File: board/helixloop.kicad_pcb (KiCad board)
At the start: 2 copper layers, 136.7 x 136.7 mm, 374 parts, among them J1 Conn_01x04, J2 Conn_01x02

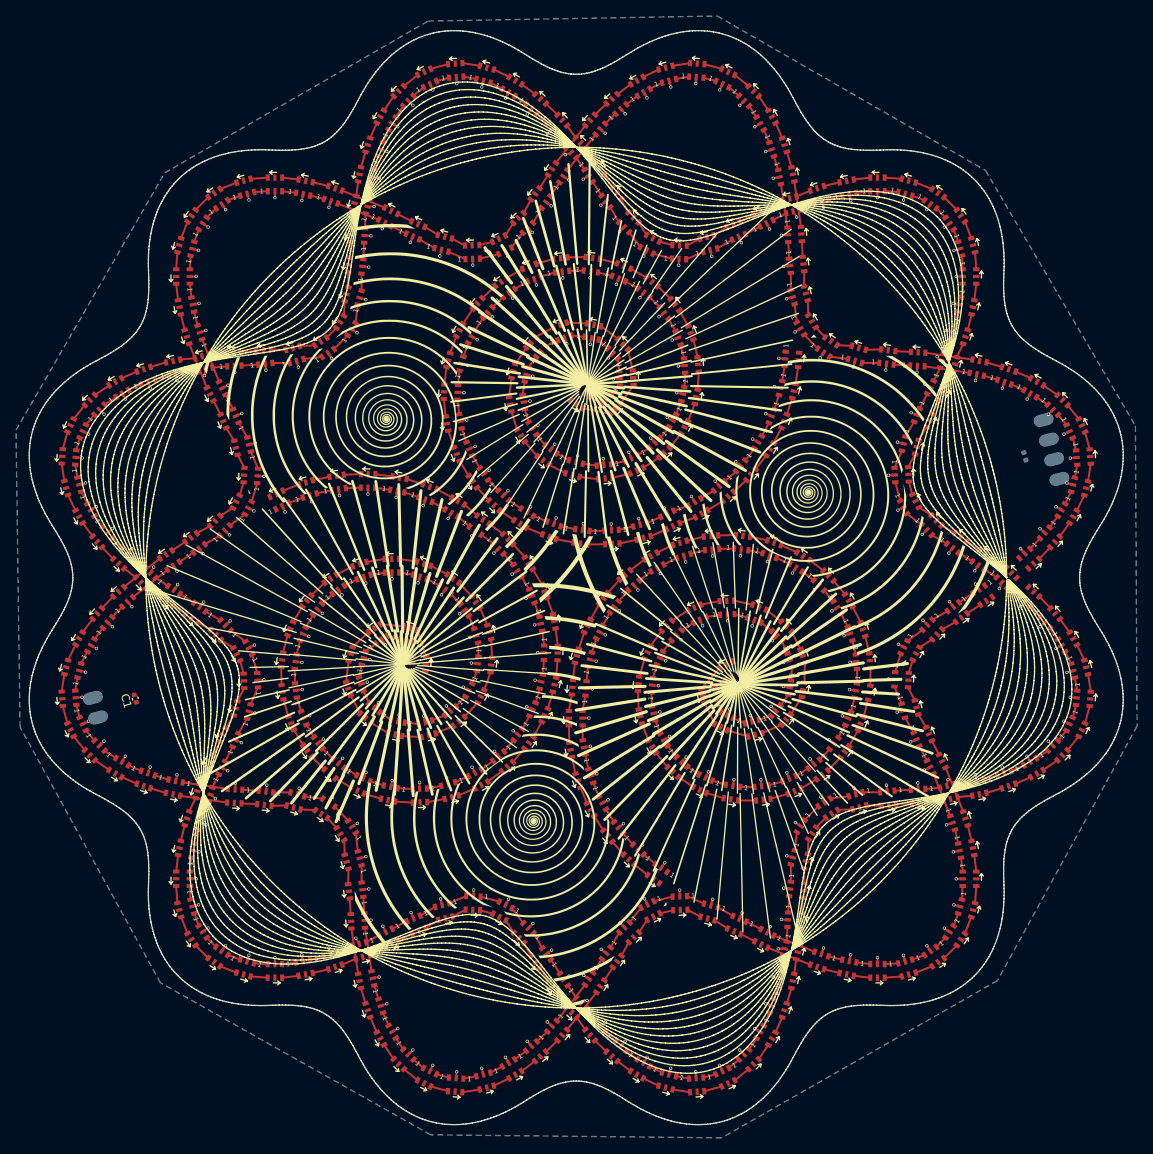
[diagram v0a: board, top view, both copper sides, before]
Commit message: draft routing
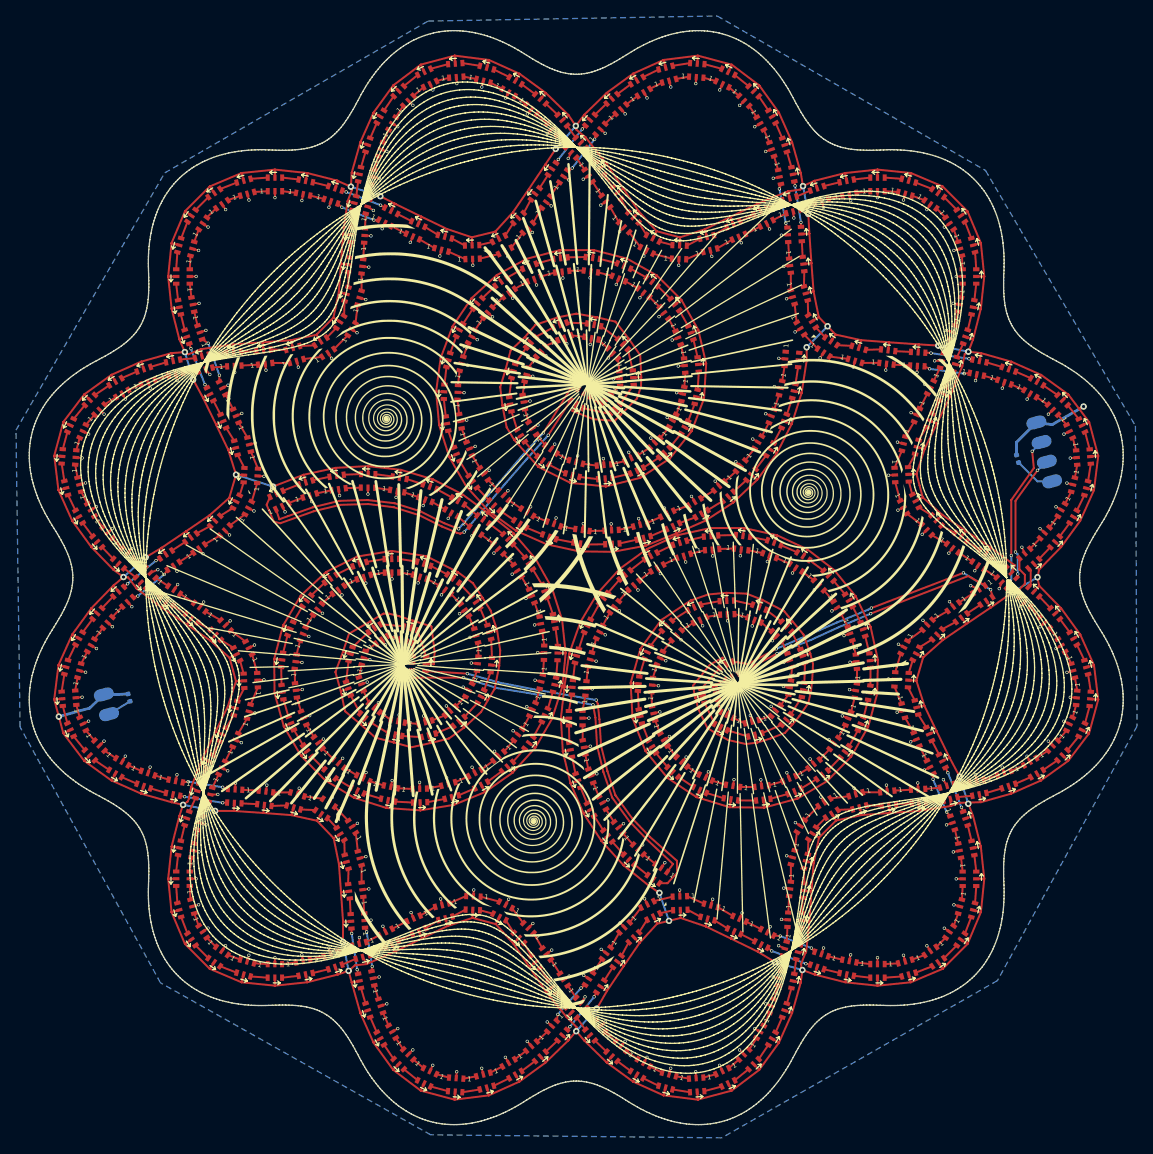
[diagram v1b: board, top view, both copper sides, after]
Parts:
- C1: moved to B.Cu
- D1, D10, D100, D101, D102, D103, D104, D105, D106, D107, D108, D109, D11, D110, D111, D112, D113, D114, D115, D116, D117, D118, D119, D12, D120, D121, D122, D123, D124, D125, D126, D127, D128, D129, D13, D130, D131, D132, D133, D134, D135, D136, D137, D138, D139, D14, D140, D141, D142, D143, D144, D145, D146, D147, D148, D149, D15, D150, D151, D152, D153, D154, D155, D156, D157, D158, D159, D16, D160, D161, D162, D163, D164, D165, D166, D167, D168, D169, D17, D170, D171, D172, D173, D174, D175, D176, D177, D178, D179, D18, D180, D181, D182, D183, D184, D185, D186, D187, D188, D189, D19, D190, D191, D192, D193, D194, D195, D196, D197, D198, D199, D2, D20, D200, D201, D202, D203, D204, D205, D206, D207, D208, D209, D21, D210, D211, D212, D213, D214, D215, D216, D217, D218, D219, D22, D220, D221, D222, D223, D224, D225, D226, D227, D228, D229, D23, D230, D231, D232, D233, D234, D235, D236, D237, D238, D239, D24, D240, D241, D242, D243, D244, D245, D246, D247, D248, D249, D25, D250, D251, D252, D253, D254, D255, D256, D257, D258, D259, D26, D260, D261, D262, D263, D264, D265, D266, D267, D268, D269, D27, D270, D271, D272, D273, D274, D275, D276, D277, D278, D279, D28, D280, D281, D282, D283, D284, D285, D286, D287, D288, D289, D29, D290, D291, D292, D293, D294, D295, D296, D297, D298, D299, D3, D30, D300, D301, D302, D303, D304, D305, D306, D307, D308, D309, D31, D310, D311, D312, D313, D314, D315, D316, D317, D318, D319, D32, D320, D321, D322, D323, D324, D325, D326, D327, D328, D329, D33, D330, D331, D332, D333, D334, D335, D336, D337, D338, D339, D34, D340, D341, D342, D343, D344, D345, D346, D347, D348, D349, D35, D350, D351, D352, D353, D354, D355, D356, D357, D358, D359, D36, D360, D361, D362, D363, D364, D365, D366, D367, D368, D369, D37, D38, D39, D4, D40, D41, D42, D43, D44, D45, D46, D47, D48, D49, D5, D50, D51, D52, D53, D54, D55, D56, D57, D58, D59, D6, D60, D61, D62, D63, D64, D65, D66, D67, D68, D69, D7, D70, D71, D72, D73, D74, D75, D76, D77, D78, D79, D8, D80, D81, D82, D83, D84, D85, D86, D87, D88, D89, D9, D90, D91, D92, D93, D94, D95, D96, D97, D98, D99: value LED-SK9822-EC20 -> SK9822-EC20
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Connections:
- D1 pad 1: (no net) -> Net-(D1-Pad1)
- D1 pad 2: (no net) -> GND
- D1 pad 3: (no net) -> /LED_SDI1
- D1 pad 4: (no net) -> /LED_CKI1
- D1 pad 5: (no net) -> +5V
- D1 pad 6: (no net) -> Net-(D1-Pad6)
- D10 pad 1: (no net) -> Net-(D10-Pad1)
- D10 pad 2: (no net) -> GND
- D10 pad 3: (no net) -> Net-(D10-Pad3)
- D10 pad 4: (no net) -> Net-(D10-Pad4)
- D10 pad 5: (no net) -> +5V
- D10 pad 6: (no net) -> Net-(D10-Pad6)
- D100 pad 1: (no net) -> Net-(D100-Pad1)
- D100 pad 2: (no net) -> GND
- D100 pad 3: (no net) -> Net-(D100-Pad3)
- D100 pad 4: (no net) -> Net-(D100-Pad4)
- D100 pad 5: (no net) -> +5V
- D100 pad 6: (no net) -> Net-(D100-Pad6)
- D101 pad 1: (no net) -> Net-(D101-Pad1)
- D101 pad 2: (no net) -> GND
- D101 pad 3: (no net) -> Net-(D100-Pad1)
- D101 pad 4: (no net) -> Net-(D100-Pad6)
- D101 pad 5: (no net) -> +5V
- D101 pad 6: (no net) -> Net-(D101-Pad6)
- D102 pad 1: (no net) -> Net-(D102-Pad1)
- D102 pad 2: (no net) -> GND
- D102 pad 3: (no net) -> Net-(D101-Pad1)
- D102 pad 4: (no net) -> Net-(D101-Pad6)
- D102 pad 5: (no net) -> +5V
- D102 pad 6: (no net) -> Net-(D102-Pad6)
- D103 pad 1: (no net) -> Net-(D103-Pad1)
- D103 pad 2: (no net) -> GND
- D103 pad 3: (no net) -> Net-(D102-Pad1)
- D103 pad 4: (no net) -> Net-(D102-Pad6)
- D103 pad 5: (no net) -> +5V
- D103 pad 6: (no net) -> Net-(D103-Pad6)
- D104 pad 1: (no net) -> Net-(D104-Pad1)
- D104 pad 2: (no net) -> GND
- D104 pad 3: (no net) -> Net-(D103-Pad1)
- D104 pad 4: (no net) -> Net-(D103-Pad6)
- D104 pad 5: (no net) -> +5V
- D104 pad 6: (no net) -> Net-(D104-Pad6)
- D105 pad 1: (no net) -> Net-(D105-Pad1)
- D105 pad 2: (no net) -> GND
- D105 pad 3: (no net) -> Net-(D104-Pad1)
- D105 pad 4: (no net) -> Net-(D104-Pad6)
- D105 pad 5: (no net) -> +5V
- D105 pad 6: (no net) -> Net-(D105-Pad6)
- D106 pad 1: (no net) -> Net-(D106-Pad1)
- D106 pad 2: (no net) -> GND
- D106 pad 3: (no net) -> Net-(D105-Pad1)
- D106 pad 4: (no net) -> Net-(D105-Pad6)
- D106 pad 5: (no net) -> +5V
- D106 pad 6: (no net) -> Net-(D106-Pad6)
- D107 pad 1: (no net) -> Net-(D107-Pad1)
- D107 pad 2: (no net) -> GND
- D107 pad 3: (no net) -> Net-(D106-Pad1)
- D107 pad 4: (no net) -> Net-(D106-Pad6)
- D107 pad 5: (no net) -> +5V
- D107 pad 6: (no net) -> Net-(D107-Pad6)
- D108 pad 1: (no net) -> Net-(D108-Pad1)
- D108 pad 2: (no net) -> GND
- D108 pad 3: (no net) -> Net-(D107-Pad1)
- D108 pad 4: (no net) -> Net-(D107-Pad6)
- D108 pad 5: (no net) -> +5V
- D108 pad 6: (no net) -> Net-(D108-Pad6)
- D109 pad 1: (no net) -> Net-(D109-Pad1)
- D109 pad 2: (no net) -> GND
- D109 pad 3: (no net) -> Net-(D108-Pad1)
- D109 pad 4: (no net) -> Net-(D108-Pad6)
- D109 pad 5: (no net) -> +5V
- D109 pad 6: (no net) -> Net-(D109-Pad6)
- D11 pad 1: (no net) -> Net-(D11-Pad1)
- D11 pad 2: (no net) -> GND
- D11 pad 3: (no net) -> Net-(D10-Pad1)
- D11 pad 4: (no net) -> Net-(D10-Pad6)
- D11 pad 5: (no net) -> +5V
- D11 pad 6: (no net) -> Net-(D11-Pad6)
- D110 pad 1: (no net) -> Net-(D110-Pad1)
- D110 pad 2: (no net) -> GND
- D110 pad 3: (no net) -> Net-(D109-Pad1)
- D110 pad 4: (no net) -> Net-(D109-Pad6)
- D110 pad 5: (no net) -> +5V
- D110 pad 6: (no net) -> Net-(D110-Pad6)
- D111 pad 1: (no net) -> Net-(D111-Pad1)
- D111 pad 2: (no net) -> GND
- D111 pad 3: (no net) -> Net-(D110-Pad1)
- D111 pad 4: (no net) -> Net-(D110-Pad6)
- D111 pad 5: (no net) -> +5V
- D111 pad 6: (no net) -> Net-(D111-Pad6)
- D112 pad 1: (no net) -> Net-(D112-Pad1)
- D112 pad 2: (no net) -> GND
- D112 pad 3: (no net) -> Net-(D111-Pad1)
- D112 pad 4: (no net) -> Net-(D111-Pad6)
- D112 pad 5: (no net) -> +5V
- D112 pad 6: (no net) -> Net-(D112-Pad6)
- D113 pad 1: (no net) -> Net-(D113-Pad1)
- D113 pad 2: (no net) -> GND
- D113 pad 3: (no net) -> Net-(D112-Pad1)
- D113 pad 4: (no net) -> Net-(D112-Pad6)
- D113 pad 5: (no net) -> +5V
- D113 pad 6: (no net) -> Net-(D113-Pad6)
- D114 pad 1: (no net) -> Net-(D114-Pad1)
- D114 pad 2: (no net) -> GND
- D114 pad 3: (no net) -> Net-(D113-Pad1)
- D114 pad 4: (no net) -> Net-(D113-Pad6)
- D114 pad 5: (no net) -> +5V
- D114 pad 6: (no net) -> Net-(D114-Pad6)
- D115 pad 1: (no net) -> Net-(D115-Pad1)
- D115 pad 2: (no net) -> GND
- D115 pad 3: (no net) -> Net-(D114-Pad1)
- D115 pad 4: (no net) -> Net-(D114-Pad6)
- D115 pad 5: (no net) -> +5V
- D115 pad 6: (no net) -> Net-(D115-Pad6)
- D116 pad 1: (no net) -> Net-(D116-Pad1)
- D116 pad 2: (no net) -> GND
- D116 pad 3: (no net) -> Net-(D115-Pad1)
- D116 pad 4: (no net) -> Net-(D115-Pad6)
- D116 pad 5: (no net) -> +5V
- D116 pad 6: (no net) -> Net-(D116-Pad6)
- D117 pad 1: (no net) -> Net-(D117-Pad1)
- D117 pad 2: (no net) -> GND
- D117 pad 3: (no net) -> Net-(D116-Pad1)
- D117 pad 4: (no net) -> Net-(D116-Pad6)
- D117 pad 5: (no net) -> +5V
- D117 pad 6: (no net) -> Net-(D117-Pad6)
- D118 pad 1: (no net) -> Net-(D118-Pad1)
- D118 pad 2: (no net) -> GND
- D118 pad 3: (no net) -> Net-(D117-Pad1)
- D118 pad 4: (no net) -> Net-(D117-Pad6)
- D118 pad 5: (no net) -> +5V
- D118 pad 6: (no net) -> Net-(D118-Pad6)
- D119 pad 1: (no net) -> Net-(D119-Pad1)
- D119 pad 2: (no net) -> GND
- D119 pad 3: (no net) -> Net-(D118-Pad1)
- D119 pad 4: (no net) -> Net-(D118-Pad6)
- D119 pad 5: (no net) -> +5V
- D119 pad 6: (no net) -> Net-(D119-Pad6)
- D12 pad 1: (no net) -> Net-(D12-Pad1)
- D12 pad 2: (no net) -> GND
- D12 pad 3: (no net) -> Net-(D11-Pad1)
- D12 pad 4: (no net) -> Net-(D11-Pad6)
- D12 pad 5: (no net) -> +5V
- D12 pad 6: (no net) -> Net-(D12-Pad6)
- D120 pad 1: (no net) -> Net-(D120-Pad1)
- D120 pad 2: (no net) -> GND
- D120 pad 3: (no net) -> Net-(D119-Pad1)
- D120 pad 4: (no net) -> Net-(D119-Pad6)
- D120 pad 5: (no net) -> +5V
- D120 pad 6: (no net) -> Net-(D120-Pad6)
- D121 pad 1: (no net) -> Net-(D121-Pad1)
- D121 pad 2: (no net) -> GND
- D121 pad 3: (no net) -> Net-(D120-Pad1)
- D121 pad 4: (no net) -> Net-(D120-Pad6)
- D121 pad 5: (no net) -> +5V
- D121 pad 6: (no net) -> Net-(D121-Pad6)
- D122 pad 1: (no net) -> Net-(D122-Pad1)
- D122 pad 2: (no net) -> GND
- D122 pad 3: (no net) -> Net-(D121-Pad1)
- D122 pad 4: (no net) -> Net-(D121-Pad6)
- D122 pad 5: (no net) -> +5V
- D122 pad 6: (no net) -> Net-(D122-Pad6)
- D123 pad 1: (no net) -> /SK9822 LED Array 1/LED_SDO
- D123 pad 2: (no net) -> GND
- D123 pad 3: (no net) -> Net-(D122-Pad1)
- D123 pad 4: (no net) -> Net-(D122-Pad6)
- D123 pad 5: (no net) -> +5V
- D123 pad 6: (no net) -> /SK9822 LED Array 1/LED_CKO
- D124 pad 1: (no net) -> Net-(D124-Pad1)
- D124 pad 2: (no net) -> GND
- D124 pad 3: (no net) -> /SK9822 LED Array 1/LED_SDO
- D124 pad 4: (no net) -> /SK9822 LED Array 1/LED_CKO
- D124 pad 5: (no net) -> +5V
- D124 pad 6: (no net) -> Net-(D124-Pad6)
- D125 pad 1: (no net) -> Net-(D125-Pad1)
- D125 pad 2: (no net) -> GND
- D125 pad 3: (no net) -> Net-(D124-Pad1)
- D125 pad 4: (no net) -> Net-(D124-Pad6)
- D125 pad 5: (no net) -> +5V
- D125 pad 6: (no net) -> Net-(D125-Pad6)
- D126 pad 1: (no net) -> Net-(D126-Pad1)
- D126 pad 2: (no net) -> GND
- D126 pad 3: (no net) -> Net-(D125-Pad1)
- D126 pad 4: (no net) -> Net-(D125-Pad6)
- D126 pad 5: (no net) -> +5V
- D126 pad 6: (no net) -> Net-(D126-Pad6)
- D127 pad 1: (no net) -> Net-(D127-Pad1)
- D127 pad 2: (no net) -> GND
- D127 pad 3: (no net) -> Net-(D126-Pad1)
- D127 pad 4: (no net) -> Net-(D126-Pad6)
- D127 pad 5: (no net) -> +5V
- D127 pad 6: (no net) -> Net-(D127-Pad6)
- D128 pad 1: (no net) -> Net-(D128-Pad1)
- D128 pad 2: (no net) -> GND
- D128 pad 3: (no net) -> Net-(D127-Pad1)
- D128 pad 4: (no net) -> Net-(D127-Pad6)
- D128 pad 5: (no net) -> +5V
- D128 pad 6: (no net) -> Net-(D128-Pad6)
- D129 pad 1: (no net) -> Net-(D129-Pad1)
- D129 pad 2: (no net) -> GND
- D129 pad 3: (no net) -> Net-(D128-Pad1)
- D129 pad 4: (no net) -> Net-(D128-Pad6)
- D129 pad 5: (no net) -> +5V
- D129 pad 6: (no net) -> Net-(D129-Pad6)
- D13 pad 1: (no net) -> Net-(D13-Pad1)
- D13 pad 2: (no net) -> GND
- D13 pad 3: (no net) -> Net-(D12-Pad1)
- D13 pad 4: (no net) -> Net-(D12-Pad6)
- D13 pad 5: (no net) -> +5V
- D13 pad 6: (no net) -> Net-(D13-Pad6)
- D130 pad 1: (no net) -> Net-(D130-Pad1)
- D130 pad 2: (no net) -> GND
- D130 pad 3: (no net) -> Net-(D129-Pad1)
- D130 pad 4: (no net) -> Net-(D129-Pad6)
- D130 pad 5: (no net) -> +5V
- D130 pad 6: (no net) -> Net-(D130-Pad6)
- D131 pad 1: (no net) -> Net-(D131-Pad1)
- D131 pad 2: (no net) -> GND
- D131 pad 3: (no net) -> Net-(D130-Pad1)
- D131 pad 4: (no net) -> Net-(D130-Pad6)
- D131 pad 5: (no net) -> +5V
- D131 pad 6: (no net) -> Net-(D131-Pad6)
- D132 pad 1: (no net) -> Net-(D132-Pad1)
- D132 pad 2: (no net) -> GND
- D132 pad 3: (no net) -> Net-(D131-Pad1)
- D132 pad 4: (no net) -> Net-(D131-Pad6)
- D132 pad 5: (no net) -> +5V
- D132 pad 6: (no net) -> Net-(D132-Pad6)
- D133 pad 1: (no net) -> Net-(D133-Pad1)
- D133 pad 2: (no net) -> GND
- D133 pad 3: (no net) -> Net-(D132-Pad1)
- D133 pad 4: (no net) -> Net-(D132-Pad6)
- D133 pad 5: (no net) -> +5V
- D133 pad 6: (no net) -> Net-(D133-Pad6)
- D134 pad 1: (no net) -> Net-(D134-Pad1)
- D134 pad 2: (no net) -> GND
- D134 pad 3: (no net) -> Net-(D133-Pad1)
- D134 pad 4: (no net) -> Net-(D133-Pad6)
- D134 pad 5: (no net) -> +5V
- D134 pad 6: (no net) -> Net-(D134-Pad6)
- D135 pad 1: (no net) -> Net-(D135-Pad1)
- D135 pad 2: (no net) -> GND
- D135 pad 3: (no net) -> Net-(D134-Pad1)
- D135 pad 4: (no net) -> Net-(D134-Pad6)
- D135 pad 5: (no net) -> +5V
- D135 pad 6: (no net) -> Net-(D135-Pad6)
- D136 pad 1: (no net) -> Net-(D136-Pad1)
- D136 pad 2: (no net) -> GND
- D136 pad 3: (no net) -> Net-(D135-Pad1)
- D136 pad 4: (no net) -> Net-(D135-Pad6)
- D136 pad 5: (no net) -> +5V
- D136 pad 6: (no net) -> Net-(D136-Pad6)
- D137 pad 1: (no net) -> Net-(D137-Pad1)
- D137 pad 2: (no net) -> GND
- D137 pad 3: (no net) -> Net-(D136-Pad1)
- D137 pad 4: (no net) -> Net-(D136-Pad6)
- D137 pad 5: (no net) -> +5V
- D137 pad 6: (no net) -> Net-(D137-Pad6)
- D138 pad 1: (no net) -> Net-(D139-Pad3)
- D138 pad 2: (no net) -> GND
- D138 pad 3: (no net) -> Net-(D137-Pad1)
- D138 pad 4: (no net) -> Net-(D137-Pad6)
- D138 pad 5: (no net) -> +5V
- D138 pad 6: (no net) -> Net-(D139-Pad4)
- D139 pad 1: (no net) -> Net-(D139-Pad1)
- D139 pad 2: (no net) -> GND
- D139 pad 3: (no net) -> Net-(D139-Pad3)
- D139 pad 4: (no net) -> Net-(D139-Pad4)
- D139 pad 5: (no net) -> +5V
- D139 pad 6: (no net) -> Net-(D139-Pad6)
- D14 pad 1: (no net) -> Net-(D14-Pad1)
- D14 pad 2: (no net) -> GND
- D14 pad 3: (no net) -> Net-(D13-Pad1)
- D14 pad 4: (no net) -> Net-(D13-Pad6)
- D14 pad 5: (no net) -> +5V
- D14 pad 6: (no net) -> Net-(D14-Pad6)
- D140 pad 1: (no net) -> Net-(D140-Pad1)
- D140 pad 2: (no net) -> GND
- D140 pad 3: (no net) -> Net-(D139-Pad1)
- D140 pad 4: (no net) -> Net-(D139-Pad6)
- D140 pad 5: (no net) -> +5V
- D140 pad 6: (no net) -> Net-(D140-Pad6)
- D141 pad 1: (no net) -> Net-(D141-Pad1)
- D141 pad 2: (no net) -> GND
- D141 pad 3: (no net) -> Net-(D140-Pad1)
- D141 pad 4: (no net) -> Net-(D140-Pad6)
- D141 pad 5: (no net) -> +5V
- D141 pad 6: (no net) -> Net-(D141-Pad6)
- D142 pad 1: (no net) -> Net-(D142-Pad1)
- D142 pad 2: (no net) -> GND
- D142 pad 3: (no net) -> Net-(D141-Pad1)
- D142 pad 4: (no net) -> Net-(D141-Pad6)
- D142 pad 5: (no net) -> +5V
- D142 pad 6: (no net) -> Net-(D142-Pad6)
- D143 pad 1: (no net) -> Net-(D143-Pad1)
- D143 pad 2: (no net) -> GND
- D143 pad 3: (no net) -> Net-(D142-Pad1)
- D143 pad 4: (no net) -> Net-(D142-Pad6)
- D143 pad 5: (no net) -> +5V
- D143 pad 6: (no net) -> Net-(D143-Pad6)
- D144 pad 1: (no net) -> Net-(D144-Pad1)
- D144 pad 2: (no net) -> GND
- D144 pad 3: (no net) -> Net-(D143-Pad1)
- D144 pad 4: (no net) -> Net-(D143-Pad6)
- D144 pad 5: (no net) -> +5V
- D144 pad 6: (no net) -> Net-(D144-Pad6)
- D145 pad 1: (no net) -> Net-(D145-Pad1)
- D145 pad 2: (no net) -> GND
- D145 pad 3: (no net) -> Net-(D144-Pad1)
- D145 pad 4: (no net) -> Net-(D144-Pad6)
- D145 pad 5: (no net) -> +5V
- D145 pad 6: (no net) -> Net-(D145-Pad6)
- D146 pad 1: (no net) -> Net-(D146-Pad1)
- D146 pad 2: (no net) -> GND
- D146 pad 3: (no net) -> Net-(D145-Pad1)
- D146 pad 4: (no net) -> Net-(D145-Pad6)
- D146 pad 5: (no net) -> +5V
- D146 pad 6: (no net) -> Net-(D146-Pad6)
- D147 pad 1: (no net) -> Net-(D147-Pad1)
- D147 pad 2: (no net) -> GND
- D147 pad 3: (no net) -> Net-(D146-Pad1)
- D147 pad 4: (no net) -> Net-(D146-Pad6)
- D147 pad 5: (no net) -> +5V
- D147 pad 6: (no net) -> Net-(D147-Pad6)
- D148 pad 1: (no net) -> Net-(D148-Pad1)
- D148 pad 2: (no net) -> GND
- D148 pad 3: (no net) -> Net-(D147-Pad1)
- D148 pad 4: (no net) -> Net-(D147-Pad6)
- D148 pad 5: (no net) -> +5V
- D148 pad 6: (no net) -> Net-(D148-Pad6)
- D149 pad 1: (no net) -> Net-(D149-Pad1)
- D149 pad 2: (no net) -> GND
- D149 pad 3: (no net) -> Net-(D148-Pad1)
- D149 pad 4: (no net) -> Net-(D148-Pad6)
- D149 pad 5: (no net) -> +5V
- D149 pad 6: (no net) -> Net-(D149-Pad6)
- D15 pad 1: (no net) -> Net-(D16-Pad3)
- D15 pad 2: (no net) -> GND
- D15 pad 3: (no net) -> Net-(D14-Pad1)
- D15 pad 4: (no net) -> Net-(D14-Pad6)
- D15 pad 5: (no net) -> +5V
- D15 pad 6: (no net) -> Net-(D16-Pad4)
- D150 pad 1: (no net) -> Net-(D150-Pad1)
- D150 pad 2: (no net) -> GND
- D150 pad 3: (no net) -> Net-(D149-Pad1)
- D150 pad 4: (no net) -> Net-(D149-Pad6)
- D150 pad 5: (no net) -> +5V
- D150 pad 6: (no net) -> Net-(D150-Pad6)
- D151 pad 1: (no net) -> Net-(D151-Pad1)
- D151 pad 2: (no net) -> GND
- D151 pad 3: (no net) -> Net-(D150-Pad1)
- D151 pad 4: (no net) -> Net-(D150-Pad6)
- D151 pad 5: (no net) -> +5V
- D151 pad 6: (no net) -> Net-(D151-Pad6)
- D152 pad 1: (no net) -> Net-(D152-Pad1)
- D152 pad 2: (no net) -> GND
- D152 pad 3: (no net) -> Net-(D151-Pad1)
- D152 pad 4: (no net) -> Net-(D151-Pad6)
- D152 pad 5: (no net) -> +5V
- D152 pad 6: (no net) -> Net-(D152-Pad6)
- D153 pad 1: (no net) -> Net-(D154-Pad3)
- D153 pad 2: (no net) -> GND
- D153 pad 3: (no net) -> Net-(D152-Pad1)
- D153 pad 4: (no net) -> Net-(D152-Pad6)
- D153 pad 5: (no net) -> +5V
- D153 pad 6: (no net) -> Net-(D154-Pad4)
- D154 pad 1: (no net) -> Net-(D154-Pad1)
- D154 pad 2: (no net) -> GND
- D154 pad 3: (no net) -> Net-(D154-Pad3)
- D154 pad 4: (no net) -> Net-(D154-Pad4)
- D154 pad 5: (no net) -> +5V
- D154 pad 6: (no net) -> Net-(D154-Pad6)
- D155 pad 1: (no net) -> Net-(D155-Pad1)
- D155 pad 2: (no net) -> GND
- D155 pad 3: (no net) -> Net-(D154-Pad1)
- D155 pad 4: (no net) -> Net-(D154-Pad6)
- D155 pad 5: (no net) -> +5V
- D155 pad 6: (no net) -> Net-(D155-Pad6)
- D156 pad 1: (no net) -> Net-(D156-Pad1)
- D156 pad 2: (no net) -> GND
- D156 pad 3: (no net) -> Net-(D155-Pad1)
- D156 pad 4: (no net) -> Net-(D155-Pad6)
- D156 pad 5: (no net) -> +5V
- D156 pad 6: (no net) -> Net-(D156-Pad6)
- D157 pad 1: (no net) -> Net-(D157-Pad1)
- D157 pad 2: (no net) -> GND
- D157 pad 3: (no net) -> Net-(D156-Pad1)
- D157 pad 4: (no net) -> Net-(D156-Pad6)
- D157 pad 5: (no net) -> +5V
- D157 pad 6: (no net) -> Net-(D157-Pad6)
- D158 pad 1: (no net) -> Net-(D158-Pad1)
- D158 pad 2: (no net) -> GND
- D158 pad 3: (no net) -> Net-(D157-Pad1)
- D158 pad 4: (no net) -> Net-(D157-Pad6)
- D158 pad 5: (no net) -> +5V
- D158 pad 6: (no net) -> Net-(D158-Pad6)
- D159 pad 1: (no net) -> Net-(D159-Pad1)
- D159 pad 2: (no net) -> GND
- D159 pad 3: (no net) -> Net-(D158-Pad1)
- D159 pad 4: (no net) -> Net-(D158-Pad6)
- D159 pad 5: (no net) -> +5V
- D159 pad 6: (no net) -> Net-(D159-Pad6)
- D16 pad 1: (no net) -> Net-(D16-Pad1)
- D16 pad 2: (no net) -> GND
- D16 pad 3: (no net) -> Net-(D16-Pad3)
- D16 pad 4: (no net) -> Net-(D16-Pad4)
- D16 pad 5: (no net) -> +5V
- D16 pad 6: (no net) -> Net-(D16-Pad6)
- D160 pad 1: (no net) -> Net-(D160-Pad1)
- D160 pad 2: (no net) -> GND
- D160 pad 3: (no net) -> Net-(D159-Pad1)
- D160 pad 4: (no net) -> Net-(D159-Pad6)
- D160 pad 5: (no net) -> +5V
- D160 pad 6: (no net) -> Net-(D160-Pad6)
- D161 pad 1: (no net) -> Net-(D161-Pad1)
- D161 pad 2: (no net) -> GND
- D161 pad 3: (no net) -> Net-(D160-Pad1)
- D161 pad 4: (no net) -> Net-(D160-Pad6)
- D161 pad 5: (no net) -> +5V
- D161 pad 6: (no net) -> Net-(D161-Pad6)
- D162 pad 1: (no net) -> Net-(D162-Pad1)
- D162 pad 2: (no net) -> GND
- D162 pad 3: (no net) -> Net-(D161-Pad1)
- D162 pad 4: (no net) -> Net-(D161-Pad6)
- D162 pad 5: (no net) -> +5V
- D162 pad 6: (no net) -> Net-(D162-Pad6)
- D163 pad 1: (no net) -> Net-(D163-Pad1)
- D163 pad 2: (no net) -> GND
- D163 pad 3: (no net) -> Net-(D162-Pad1)
- D163 pad 4: (no net) -> Net-(D162-Pad6)
- D163 pad 5: (no net) -> +5V
- D163 pad 6: (no net) -> Net-(D163-Pad6)
- D164 pad 1: (no net) -> Net-(D164-Pad1)
- D164 pad 2: (no net) -> GND
- D164 pad 3: (no net) -> Net-(D163-Pad1)
- D164 pad 4: (no net) -> Net-(D163-Pad6)
- D164 pad 5: (no net) -> +5V
- D164 pad 6: (no net) -> Net-(D164-Pad6)
- D165 pad 1: (no net) -> Net-(D165-Pad1)
- D165 pad 2: (no net) -> GND
- D165 pad 3: (no net) -> Net-(D164-Pad1)
- D165 pad 4: (no net) -> Net-(D164-Pad6)
- D165 pad 5: (no net) -> +5V
- D165 pad 6: (no net) -> Net-(D165-Pad6)
- D166 pad 1: (no net) -> Net-(D166-Pad1)
- D166 pad 2: (no net) -> GND
- D166 pad 3: (no net) -> Net-(D165-Pad1)
- D166 pad 4: (no net) -> Net-(D165-Pad6)
- D166 pad 5: (no net) -> +5V
- D166 pad 6: (no net) -> Net-(D166-Pad6)
- D167 pad 1: (no net) -> Net-(D167-Pad1)
- D167 pad 2: (no net) -> GND
- D167 pad 3: (no net) -> Net-(D166-Pad1)
- D167 pad 4: (no net) -> Net-(D166-Pad6)
- D167 pad 5: (no net) -> +5V
- D167 pad 6: (no net) -> Net-(D167-Pad6)
- D168 pad 1: (no net) -> Net-(D168-Pad1)
- D168 pad 2: (no net) -> GND
- D168 pad 3: (no net) -> Net-(D167-Pad1)
- D168 pad 4: (no net) -> Net-(D167-Pad6)
- D168 pad 5: (no net) -> +5V
- D168 pad 6: (no net) -> Net-(D168-Pad6)
- D169 pad 1: (no net) -> Net-(D169-Pad1)
- D169 pad 2: (no net) -> GND
- D169 pad 3: (no net) -> Net-(D168-Pad1)
- D169 pad 4: (no net) -> Net-(D168-Pad6)
- D169 pad 5: (no net) -> +5V
- D169 pad 6: (no net) -> Net-(D169-Pad6)
- D17 pad 1: (no net) -> Net-(D17-Pad1)
- D17 pad 2: (no net) -> GND
- D17 pad 3: (no net) -> Net-(D16-Pad1)
- D17 pad 4: (no net) -> Net-(D16-Pad6)
- D17 pad 5: (no net) -> +5V
- D17 pad 6: (no net) -> Net-(D17-Pad6)
- D170 pad 1: (no net) -> Net-(D170-Pad1)
- D170 pad 2: (no net) -> GND
- D170 pad 3: (no net) -> Net-(D169-Pad1)
- D170 pad 4: (no net) -> Net-(D169-Pad6)
- D170 pad 5: (no net) -> +5V
- D170 pad 6: (no net) -> Net-(D170-Pad6)
- D171 pad 1: (no net) -> Net-(D171-Pad1)
- D171 pad 2: (no net) -> GND
- D171 pad 3: (no net) -> Net-(D170-Pad1)
- D171 pad 4: (no net) -> Net-(D170-Pad6)
- D171 pad 5: (no net) -> +5V
- D171 pad 6: (no net) -> Net-(D171-Pad6)
- D172 pad 1: (no net) -> Net-(D172-Pad1)
- D172 pad 2: (no net) -> GND
- D172 pad 3: (no net) -> Net-(D171-Pad1)
- D172 pad 4: (no net) -> Net-(D171-Pad6)
- D172 pad 5: (no net) -> +5V
- D172 pad 6: (no net) -> Net-(D172-Pad6)
- D173 pad 1: (no net) -> Net-(D173-Pad1)
- D173 pad 2: (no net) -> GND
- D173 pad 3: (no net) -> Net-(D172-Pad1)
- D173 pad 4: (no net) -> Net-(D172-Pad6)
- D173 pad 5: (no net) -> +5V
- D173 pad 6: (no net) -> Net-(D173-Pad6)
- D174 pad 1: (no net) -> Net-(D174-Pad1)
- D174 pad 2: (no net) -> GND
- D174 pad 3: (no net) -> Net-(D173-Pad1)
- D174 pad 4: (no net) -> Net-(D173-Pad6)
- D174 pad 5: (no net) -> +5V
- D174 pad 6: (no net) -> Net-(D174-Pad6)
- D175 pad 1: (no net) -> Net-(D175-Pad1)
- D175 pad 2: (no net) -> GND
- D175 pad 3: (no net) -> Net-(D174-Pad1)
- D175 pad 4: (no net) -> Net-(D174-Pad6)
- D175 pad 5: (no net) -> +5V
- D175 pad 6: (no net) -> Net-(D175-Pad6)
- D176 pad 1: (no net) -> Net-(D176-Pad1)
- D176 pad 2: (no net) -> GND
- D176 pad 3: (no net) -> Net-(D175-Pad1)
- D176 pad 4: (no net) -> Net-(D175-Pad6)
- D176 pad 5: (no net) -> +5V
- D176 pad 6: (no net) -> Net-(D176-Pad6)
- D177 pad 1: (no net) -> Net-(D177-Pad1)
- D177 pad 2: (no net) -> GND
- D177 pad 3: (no net) -> Net-(D176-Pad1)
- D177 pad 4: (no net) -> Net-(D176-Pad6)
- D177 pad 5: (no net) -> +5V
- D177 pad 6: (no net) -> Net-(D177-Pad6)
- D178 pad 1: (no net) -> Net-(D178-Pad1)
- D178 pad 2: (no net) -> GND
- D178 pad 3: (no net) -> Net-(D177-Pad1)
- D178 pad 4: (no net) -> Net-(D177-Pad6)
- D178 pad 5: (no net) -> +5V
- D178 pad 6: (no net) -> Net-(D178-Pad6)
- D179 pad 1: (no net) -> Net-(D179-Pad1)
- D179 pad 2: (no net) -> GND
- D179 pad 3: (no net) -> Net-(D178-Pad1)
- D179 pad 4: (no net) -> Net-(D178-Pad6)
- D179 pad 5: (no net) -> +5V
- D179 pad 6: (no net) -> Net-(D179-Pad6)
- D18 pad 1: (no net) -> Net-(D18-Pad1)
- D18 pad 2: (no net) -> GND
- D18 pad 3: (no net) -> Net-(D17-Pad1)
- D18 pad 4: (no net) -> Net-(D17-Pad6)
- D18 pad 5: (no net) -> +5V
- D18 pad 6: (no net) -> Net-(D18-Pad6)
- D180 pad 1: (no net) -> Net-(D180-Pad1)
- D180 pad 2: (no net) -> GND
- D180 pad 3: (no net) -> Net-(D179-Pad1)
- D180 pad 4: (no net) -> Net-(D179-Pad6)
- D180 pad 5: (no net) -> +5V
- D180 pad 6: (no net) -> Net-(D180-Pad6)
- D181 pad 1: (no net) -> Net-(D181-Pad1)
- D181 pad 2: (no net) -> GND
- D181 pad 3: (no net) -> Net-(D180-Pad1)
- D181 pad 4: (no net) -> Net-(D180-Pad6)
- D181 pad 5: (no net) -> +5V
- D181 pad 6: (no net) -> Net-(D181-Pad6)
- D182 pad 1: (no net) -> Net-(D182-Pad1)
- D182 pad 2: (no net) -> GND
- D182 pad 3: (no net) -> Net-(D181-Pad1)
- D182 pad 4: (no net) -> Net-(D181-Pad6)
- D182 pad 5: (no net) -> +5V
- D182 pad 6: (no net) -> Net-(D182-Pad6)
- D183 pad 1: (no net) -> Net-(D184-Pad3)
- D183 pad 2: (no net) -> GND
- D183 pad 3: (no net) -> Net-(D182-Pad1)
- D183 pad 4: (no net) -> Net-(D182-Pad6)
- D183 pad 5: (no net) -> +5V
- D183 pad 6: (no net) -> Net-(D184-Pad4)
- D184 pad 1: (no net) -> Net-(D184-Pad1)
- D184 pad 2: (no net) -> GND
- D184 pad 3: (no net) -> Net-(D184-Pad3)
- D184 pad 4: (no net) -> Net-(D184-Pad4)
- D184 pad 5: (no net) -> +5V
- D184 pad 6: (no net) -> Net-(D184-Pad6)
- D185 pad 1: (no net) -> Net-(D185-Pad1)
- D185 pad 2: (no net) -> GND
- D185 pad 3: (no net) -> Net-(D184-Pad1)
- D185 pad 4: (no net) -> Net-(D184-Pad6)
- D185 pad 5: (no net) -> +5V
- D185 pad 6: (no net) -> Net-(D185-Pad6)
- D186 pad 1: (no net) -> Net-(D186-Pad1)
- D186 pad 2: (no net) -> GND
- D186 pad 3: (no net) -> Net-(D185-Pad1)
- D186 pad 4: (no net) -> Net-(D185-Pad6)
- D186 pad 5: (no net) -> +5V
- D186 pad 6: (no net) -> Net-(D186-Pad6)
- D187 pad 1: (no net) -> Net-(D187-Pad1)
- D187 pad 2: (no net) -> GND
- D187 pad 3: (no net) -> Net-(D186-Pad1)
- D187 pad 4: (no net) -> Net-(D186-Pad6)
- D187 pad 5: (no net) -> +5V
- D187 pad 6: (no net) -> Net-(D187-Pad6)
- D188 pad 1: (no net) -> Net-(D188-Pad1)
- D188 pad 2: (no net) -> GND
- D188 pad 3: (no net) -> Net-(D187-Pad1)
- D188 pad 4: (no net) -> Net-(D187-Pad6)
- D188 pad 5: (no net) -> +5V
- D188 pad 6: (no net) -> Net-(D188-Pad6)
- D189 pad 1: (no net) -> Net-(D189-Pad1)
- D189 pad 2: (no net) -> GND
- D189 pad 3: (no net) -> Net-(D188-Pad1)
- D189 pad 4: (no net) -> Net-(D188-Pad6)
- D189 pad 5: (no net) -> +5V
- D189 pad 6: (no net) -> Net-(D189-Pad6)
- D19 pad 1: (no net) -> Net-(D19-Pad1)
- D19 pad 2: (no net) -> GND
- D19 pad 3: (no net) -> Net-(D18-Pad1)
- D19 pad 4: (no net) -> Net-(D18-Pad6)
- D19 pad 5: (no net) -> +5V
- D19 pad 6: (no net) -> Net-(D19-Pad6)
- D190 pad 1: (no net) -> Net-(D190-Pad1)
- D190 pad 2: (no net) -> GND
- D190 pad 3: (no net) -> Net-(D189-Pad1)
- D190 pad 4: (no net) -> Net-(D189-Pad6)
- D190 pad 5: (no net) -> +5V
- D190 pad 6: (no net) -> Net-(D190-Pad6)
- D191 pad 1: (no net) -> Net-(D191-Pad1)
- D191 pad 2: (no net) -> GND
- D191 pad 3: (no net) -> Net-(D190-Pad1)
- D191 pad 4: (no net) -> Net-(D190-Pad6)
- D191 pad 5: (no net) -> +5V
- D191 pad 6: (no net) -> Net-(D191-Pad6)
- D192 pad 1: (no net) -> Net-(D192-Pad1)
- D192 pad 2: (no net) -> GND
- D192 pad 3: (no net) -> Net-(D191-Pad1)
- D192 pad 4: (no net) -> Net-(D191-Pad6)
- D192 pad 5: (no net) -> +5V
- D192 pad 6: (no net) -> Net-(D192-Pad6)
- D193 pad 1: (no net) -> Net-(D193-Pad1)
- D193 pad 2: (no net) -> GND
- D193 pad 3: (no net) -> Net-(D192-Pad1)
- D193 pad 4: (no net) -> Net-(D192-Pad6)
- D193 pad 5: (no net) -> +5V
- D193 pad 6: (no net) -> Net-(D193-Pad6)
- D194 pad 1: (no net) -> Net-(D194-Pad1)
- D194 pad 2: (no net) -> GND
- D194 pad 3: (no net) -> Net-(D193-Pad1)
- D194 pad 4: (no net) -> Net-(D193-Pad6)
- D194 pad 5: (no net) -> +5V
- D194 pad 6: (no net) -> Net-(D194-Pad6)
- D195 pad 1: (no net) -> Net-(D195-Pad1)
- D195 pad 2: (no net) -> GND
- D195 pad 3: (no net) -> Net-(D194-Pad1)
- D195 pad 4: (no net) -> Net-(D194-Pad6)
- D195 pad 5: (no net) -> +5V
- D195 pad 6: (no net) -> Net-(D195-Pad6)
- D196 pad 1: (no net) -> Net-(D196-Pad1)
- D196 pad 2: (no net) -> GND
- D196 pad 3: (no net) -> Net-(D195-Pad1)
- D196 pad 4: (no net) -> Net-(D195-Pad6)
- D196 pad 5: (no net) -> +5V
- D196 pad 6: (no net) -> Net-(D196-Pad6)
- D197 pad 1: (no net) -> Net-(D197-Pad1)
- D197 pad 2: (no net) -> GND
- D197 pad 3: (no net) -> Net-(D196-Pad1)
- D197 pad 4: (no net) -> Net-(D196-Pad6)
- D197 pad 5: (no net) -> +5V
- D197 pad 6: (no net) -> Net-(D197-Pad6)
- D198 pad 1: (no net) -> Net-(D198-Pad1)
- D198 pad 2: (no net) -> GND
- D198 pad 3: (no net) -> Net-(D197-Pad1)
- D198 pad 4: (no net) -> Net-(D197-Pad6)
- D198 pad 5: (no net) -> +5V
- D198 pad 6: (no net) -> Net-(D198-Pad6)
- D199 pad 1: (no net) -> Net-(D199-Pad1)
- D199 pad 2: (no net) -> GND
- D199 pad 3: (no net) -> Net-(D198-Pad1)
- D199 pad 4: (no net) -> Net-(D198-Pad6)
- D199 pad 5: (no net) -> +5V
- D199 pad 6: (no net) -> Net-(D199-Pad6)
- D2 pad 1: (no net) -> Net-(D2-Pad1)
- D2 pad 2: (no net) -> GND
- D2 pad 3: (no net) -> Net-(D1-Pad1)
- D2 pad 4: (no net) -> Net-(D1-Pad6)
- D2 pad 5: (no net) -> +5V
- D2 pad 6: (no net) -> Net-(D2-Pad6)
- D20 pad 1: (no net) -> Net-(D20-Pad1)
- D20 pad 2: (no net) -> GND
- D20 pad 3: (no net) -> Net-(D19-Pad1)
- D20 pad 4: (no net) -> Net-(D19-Pad6)
- D20 pad 5: (no net) -> +5V
- D20 pad 6: (no net) -> Net-(D20-Pad6)
- D200 pad 1: (no net) -> Net-(D200-Pad1)
- D200 pad 2: (no net) -> GND
- D200 pad 3: (no net) -> Net-(D199-Pad1)
- D200 pad 4: (no net) -> Net-(D199-Pad6)
- D200 pad 5: (no net) -> +5V
- D200 pad 6: (no net) -> Net-(D200-Pad6)
- D201 pad 1: (no net) -> Net-(D201-Pad1)
- D201 pad 2: (no net) -> GND
- D201 pad 3: (no net) -> Net-(D200-Pad1)
- D201 pad 4: (no net) -> Net-(D200-Pad6)
- D201 pad 5: (no net) -> +5V
- D201 pad 6: (no net) -> Net-(D201-Pad6)
- D202 pad 1: (no net) -> Net-(D202-Pad1)
- D202 pad 2: (no net) -> GND
- D202 pad 3: (no net) -> Net-(D201-Pad1)
- D202 pad 4: (no net) -> Net-(D201-Pad6)
- D202 pad 5: (no net) -> +5V
- D202 pad 6: (no net) -> Net-(D202-Pad6)
- D203 pad 1: (no net) -> Net-(D203-Pad1)
- D203 pad 2: (no net) -> GND
- D203 pad 3: (no net) -> Net-(D202-Pad1)
- D203 pad 4: (no net) -> Net-(D202-Pad6)
- D203 pad 5: (no net) -> +5V
- D203 pad 6: (no net) -> Net-(D203-Pad6)
- D204 pad 1: (no net) -> Net-(D204-Pad1)
- D204 pad 2: (no net) -> GND
- D204 pad 3: (no net) -> Net-(D203-Pad1)
- D204 pad 4: (no net) -> Net-(D203-Pad6)
- D204 pad 5: (no net) -> +5V
- D204 pad 6: (no net) -> Net-(D204-Pad6)
- D205 pad 1: (no net) -> Net-(D205-Pad1)
- D205 pad 2: (no net) -> GND
- D205 pad 3: (no net) -> Net-(D204-Pad1)
- D205 pad 4: (no net) -> Net-(D204-Pad6)
- D205 pad 5: (no net) -> +5V
- D205 pad 6: (no net) -> Net-(D205-Pad6)
- D206 pad 1: (no net) -> Net-(D206-Pad1)
- D206 pad 2: (no net) -> GND
- D206 pad 3: (no net) -> Net-(D205-Pad1)
- D206 pad 4: (no net) -> Net-(D205-Pad6)
- D206 pad 5: (no net) -> +5V
- D206 pad 6: (no net) -> Net-(D206-Pad6)
- D207 pad 1: (no net) -> Net-(D207-Pad1)
- D207 pad 2: (no net) -> GND
- D207 pad 3: (no net) -> Net-(D206-Pad1)
- D207 pad 4: (no net) -> Net-(D206-Pad6)
- D207 pad 5: (no net) -> +5V
- D207 pad 6: (no net) -> Net-(D207-Pad6)
- D208 pad 1: (no net) -> Net-(D208-Pad1)
- D208 pad 2: (no net) -> GND
- D208 pad 3: (no net) -> Net-(D207-Pad1)
- D208 pad 4: (no net) -> Net-(D207-Pad6)
- D208 pad 5: (no net) -> +5V
- D208 pad 6: (no net) -> Net-(D208-Pad6)
- D209 pad 1: (no net) -> Net-(D209-Pad1)
- D209 pad 2: (no net) -> GND
- D209 pad 3: (no net) -> Net-(D208-Pad1)
- D209 pad 4: (no net) -> Net-(D208-Pad6)
- D209 pad 5: (no net) -> +5V
- D209 pad 6: (no net) -> Net-(D209-Pad6)
- D21 pad 1: (no net) -> Net-(D21-Pad1)
- D21 pad 2: (no net) -> GND
- D21 pad 3: (no net) -> Net-(D20-Pad1)
- D21 pad 4: (no net) -> Net-(D20-Pad6)
- D21 pad 5: (no net) -> +5V
- D21 pad 6: (no net) -> Net-(D21-Pad6)
- D210 pad 1: (no net) -> Net-(D210-Pad1)
- D210 pad 2: (no net) -> GND
- D210 pad 3: (no net) -> Net-(D209-Pad1)
- D210 pad 4: (no net) -> Net-(D209-Pad6)
- D210 pad 5: (no net) -> +5V
- D210 pad 6: (no net) -> Net-(D210-Pad6)
- D211 pad 1: (no net) -> Net-(D211-Pad1)
- D211 pad 2: (no net) -> GND
- D211 pad 3: (no net) -> Net-(D210-Pad1)
- D211 pad 4: (no net) -> Net-(D210-Pad6)
- D211 pad 5: (no net) -> +5V
- D211 pad 6: (no net) -> Net-(D211-Pad6)
- D212 pad 1: (no net) -> Net-(D212-Pad1)
- D212 pad 2: (no net) -> GND
- D212 pad 3: (no net) -> Net-(D211-Pad1)
- D212 pad 4: (no net) -> Net-(D211-Pad6)
- D212 pad 5: (no net) -> +5V
- D212 pad 6: (no net) -> Net-(D212-Pad6)
- D213 pad 1: (no net) -> Net-(D213-Pad1)
- D213 pad 2: (no net) -> GND
- D213 pad 3: (no net) -> Net-(D212-Pad1)
- D213 pad 4: (no net) -> Net-(D212-Pad6)
- D213 pad 5: (no net) -> +5V
- D213 pad 6: (no net) -> Net-(D213-Pad6)
- D214 pad 1: (no net) -> Net-(D214-Pad1)
- D214 pad 2: (no net) -> GND
- D214 pad 3: (no net) -> Net-(D213-Pad1)
- D214 pad 4: (no net) -> Net-(D213-Pad6)
- D214 pad 5: (no net) -> +5V
- D214 pad 6: (no net) -> Net-(D214-Pad6)
- D215 pad 1: (no net) -> Net-(D215-Pad1)
- D215 pad 2: (no net) -> GND
- D215 pad 3: (no net) -> Net-(D214-Pad1)
- D215 pad 4: (no net) -> Net-(D214-Pad6)
- D215 pad 5: (no net) -> +5V
- D215 pad 6: (no net) -> Net-(D215-Pad6)
- D216 pad 1: (no net) -> Net-(D216-Pad1)
- D216 pad 2: (no net) -> GND
- D216 pad 3: (no net) -> Net-(D215-Pad1)
- D216 pad 4: (no net) -> Net-(D215-Pad6)
- D216 pad 5: (no net) -> +5V
- D216 pad 6: (no net) -> Net-(D216-Pad6)
- D217 pad 1: (no net) -> Net-(D217-Pad1)
- D217 pad 2: (no net) -> GND
- D217 pad 3: (no net) -> Net-(D216-Pad1)
- D217 pad 4: (no net) -> Net-(D216-Pad6)
- D217 pad 5: (no net) -> +5V
- D217 pad 6: (no net) -> Net-(D217-Pad6)
- D218 pad 1: (no net) -> Net-(D218-Pad1)
- D218 pad 2: (no net) -> GND
- D218 pad 3: (no net) -> Net-(D217-Pad1)
- D218 pad 4: (no net) -> Net-(D217-Pad6)
- D218 pad 5: (no net) -> +5V
- D218 pad 6: (no net) -> Net-(D218-Pad6)
- D219 pad 1: (no net) -> Net-(D219-Pad1)
- D219 pad 2: (no net) -> GND
- D219 pad 3: (no net) -> Net-(D218-Pad1)
- D219 pad 4: (no net) -> Net-(D218-Pad6)
- D219 pad 5: (no net) -> +5V
- D219 pad 6: (no net) -> Net-(D219-Pad6)
- D22 pad 1: (no net) -> Net-(D22-Pad1)
- D22 pad 2: (no net) -> GND
- D22 pad 3: (no net) -> Net-(D21-Pad1)
- D22 pad 4: (no net) -> Net-(D21-Pad6)
- D22 pad 5: (no net) -> +5V
- D22 pad 6: (no net) -> Net-(D22-Pad6)
- D220 pad 1: (no net) -> Net-(D220-Pad1)
- D220 pad 2: (no net) -> GND
- D220 pad 3: (no net) -> Net-(D219-Pad1)
- D220 pad 4: (no net) -> Net-(D219-Pad6)
- D220 pad 5: (no net) -> +5V
- D220 pad 6: (no net) -> Net-(D220-Pad6)
- D221 pad 1: (no net) -> Net-(D221-Pad1)
- D221 pad 2: (no net) -> GND
- D221 pad 3: (no net) -> Net-(D220-Pad1)
- D221 pad 4: (no net) -> Net-(D220-Pad6)
- D221 pad 5: (no net) -> +5V
- D221 pad 6: (no net) -> Net-(D221-Pad6)
- D222 pad 1: (no net) -> Net-(D222-Pad1)
- D222 pad 2: (no net) -> GND
- D222 pad 3: (no net) -> Net-(D221-Pad1)
- D222 pad 4: (no net) -> Net-(D221-Pad6)
- D222 pad 5: (no net) -> +5V
- D222 pad 6: (no net) -> Net-(D222-Pad6)
- D223 pad 1: (no net) -> Net-(D223-Pad1)
- D223 pad 2: (no net) -> GND
- D223 pad 3: (no net) -> Net-(D222-Pad1)
- D223 pad 4: (no net) -> Net-(D222-Pad6)
- D223 pad 5: (no net) -> +5V
- D223 pad 6: (no net) -> Net-(D223-Pad6)
- D224 pad 1: (no net) -> Net-(D224-Pad1)
- D224 pad 2: (no net) -> GND
- D224 pad 3: (no net) -> Net-(D223-Pad1)
- D224 pad 4: (no net) -> Net-(D223-Pad6)
- D224 pad 5: (no net) -> +5V
- D224 pad 6: (no net) -> Net-(D224-Pad6)
- D225 pad 1: (no net) -> Net-(D225-Pad1)
- D225 pad 2: (no net) -> GND
- D225 pad 3: (no net) -> Net-(D224-Pad1)
- D225 pad 4: (no net) -> Net-(D224-Pad6)
- D225 pad 5: (no net) -> +5V
- D225 pad 6: (no net) -> Net-(D225-Pad6)
- D226 pad 1: (no net) -> Net-(D226-Pad1)
- D226 pad 2: (no net) -> GND
- D226 pad 3: (no net) -> Net-(D225-Pad1)
- D226 pad 4: (no net) -> Net-(D225-Pad6)
- D226 pad 5: (no net) -> +5V
- D226 pad 6: (no net) -> Net-(D226-Pad6)
- D227 pad 1: (no net) -> Net-(D227-Pad1)
- D227 pad 2: (no net) -> GND
- D227 pad 3: (no net) -> Net-(D226-Pad1)
- D227 pad 4: (no net) -> Net-(D226-Pad6)
- D227 pad 5: (no net) -> +5V
- D227 pad 6: (no net) -> Net-(D227-Pad6)
- D228 pad 1: (no net) -> Net-(D228-Pad1)
- D228 pad 2: (no net) -> GND
- D228 pad 3: (no net) -> Net-(D227-Pad1)
- D228 pad 4: (no net) -> Net-(D227-Pad6)
- D228 pad 5: (no net) -> +5V
- D228 pad 6: (no net) -> Net-(D228-Pad6)
- D229 pad 1: (no net) -> Net-(D229-Pad1)
- D229 pad 2: (no net) -> GND
- D229 pad 3: (no net) -> Net-(D228-Pad1)
- D229 pad 4: (no net) -> Net-(D228-Pad6)
- D229 pad 5: (no net) -> +5V
- D229 pad 6: (no net) -> Net-(D229-Pad6)
- D23 pad 1: (no net) -> Net-(D23-Pad1)
- D23 pad 2: (no net) -> GND
- D23 pad 3: (no net) -> Net-(D22-Pad1)
- D23 pad 4: (no net) -> Net-(D22-Pad6)
- D23 pad 5: (no net) -> +5V
- D23 pad 6: (no net) -> Net-(D23-Pad6)
- D230 pad 1: (no net) -> Net-(D230-Pad1)
- D230 pad 2: (no net) -> GND
- D230 pad 3: (no net) -> Net-(D229-Pad1)
- D230 pad 4: (no net) -> Net-(D229-Pad6)
- D230 pad 5: (no net) -> +5V
- D230 pad 6: (no net) -> Net-(D230-Pad6)
- D231 pad 1: (no net) -> Net-(D231-Pad1)
- D231 pad 2: (no net) -> GND
- D231 pad 3: (no net) -> Net-(D230-Pad1)
- D231 pad 4: (no net) -> Net-(D230-Pad6)
- D231 pad 5: (no net) -> +5V
- D231 pad 6: (no net) -> Net-(D231-Pad6)
- D232 pad 1: (no net) -> Net-(D232-Pad1)
- D232 pad 2: (no net) -> GND
- D232 pad 3: (no net) -> Net-(D231-Pad1)
- D232 pad 4: (no net) -> Net-(D231-Pad6)
- D232 pad 5: (no net) -> +5V
- D232 pad 6: (no net) -> Net-(D232-Pad6)
- D233 pad 1: (no net) -> Net-(D233-Pad1)
- D233 pad 2: (no net) -> GND
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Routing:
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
